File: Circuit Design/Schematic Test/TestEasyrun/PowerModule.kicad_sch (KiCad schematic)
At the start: 33 parts

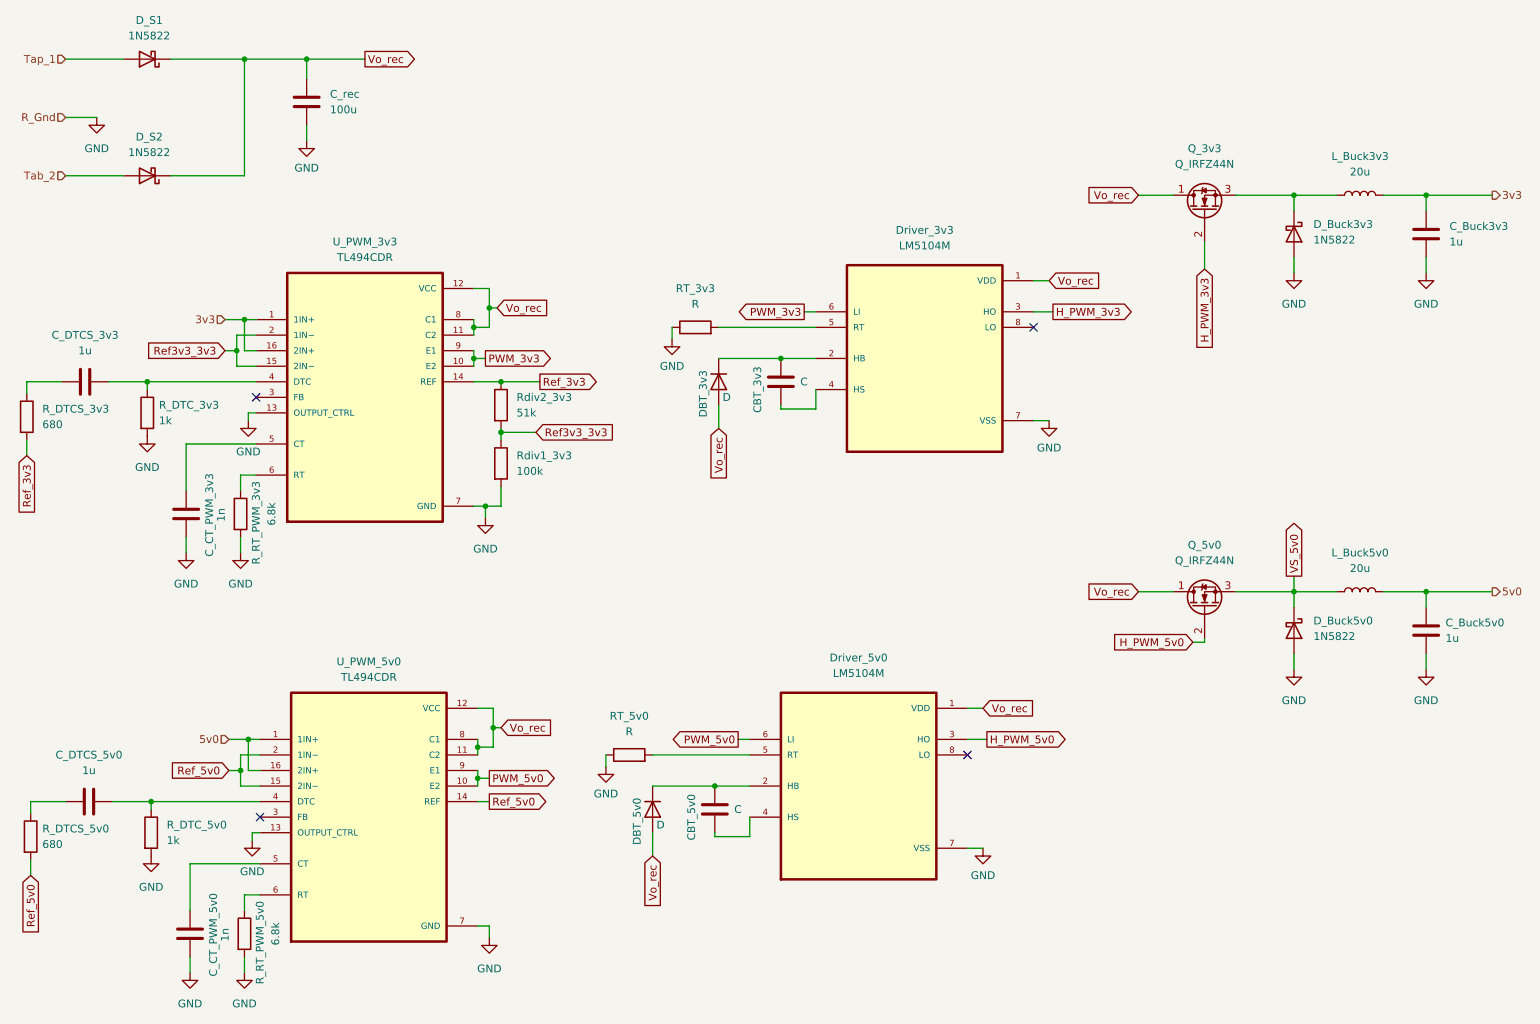
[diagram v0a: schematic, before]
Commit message: PWM generator file
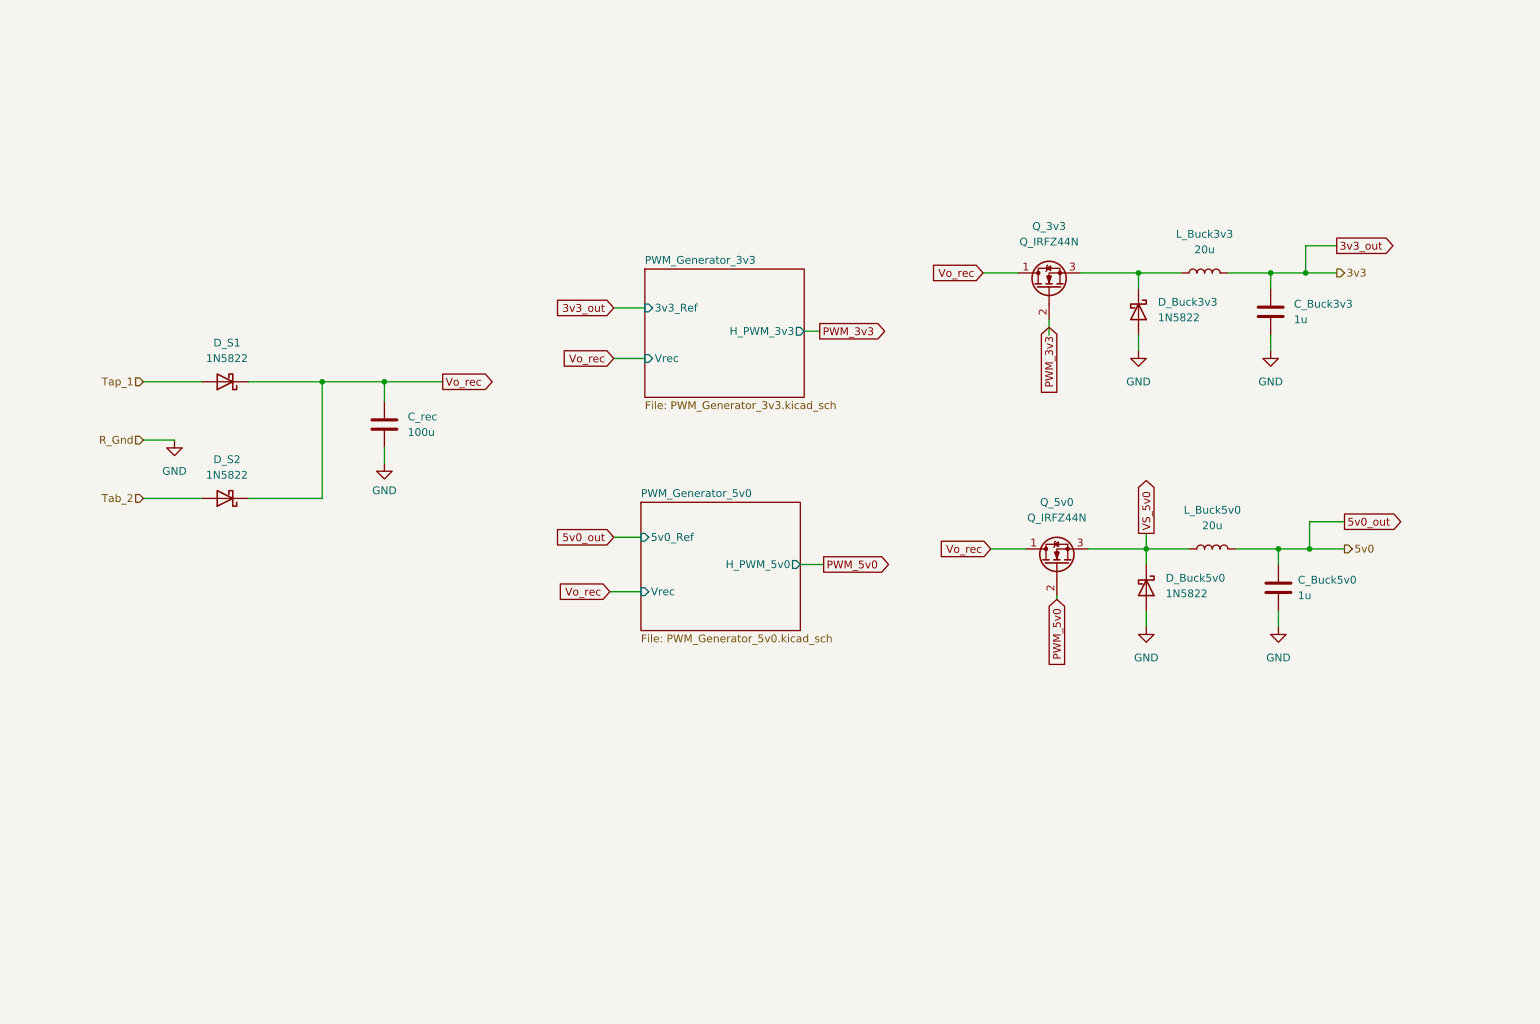
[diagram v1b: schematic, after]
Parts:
- removed CBT_3v3, CBT_5v0: C, Capacitor_SMD:C_0805_2012Metric_Pad1.18x1.45mm_HandSolder, symbol Device:C
- removed C_CT_PWM_3v3, C_CT_PWM_5v0: 1n, Capacitor_SMD:C_0805_2012Metric_Pad1.18x1.45mm_HandSolder, symbol Device:C
- removed C_DTCS_3v3, C_DTCS_5v0: 1u, Capacitor_SMD:C_0805_2012Metric_Pad1.18x1.45mm_HandSolder, symbol Device:C
- removed DBT_3v3, DBT_5v0: D, Diode_THT:D_DO-201AD_P15.24mm_Horizontal, symbol Device:D
- removed Driver_3v3, Driver_5v0: LM5104M, LM5104M:SOIC127P599X175-8N, symbol LM5104M:LM5104M
- removed RT_3v3, RT_5v0: R, Resistor_SMD:R_0805_2012Metric_Pad1.20x1.40mm_HandSolder, symbol Device:R
- removed R_DTCS_3v3, R_DTCS_5v0: 680, Resistor_SMD:R_0805_2012Metric_Pad1.20x1.40mm_HandSolder, symbol Device:R
- removed R_DTC_3v3, R_DTC_5v0: 1k, Resistor_SMD:R_0805_2012Metric_Pad1.20x1.40mm_HandSolder, symbol Device:R
- removed R_RT_PWM_3v3, R_RT_PWM_5v0: 6.8k, Resistor_SMD:R_0805_2012Metric_Pad1.20x1.40mm_HandSolder, symbol Device:R
- removed Rdiv1_3v3: 100k, Resistor_SMD:R_0805_2012Metric_Pad1.20x1.40mm_HandSolder, symbol Device:R
- removed Rdiv2_3v3: 51k, Resistor_SMD:R_0805_2012Metric_Pad1.20x1.40mm_HandSolder, symbol Device:R
- removed U_PWM_3v3, U_PWM_5v0: TL494CDR, TL494CDR_PWM:SOIC127P600X175-16N, symbol TL494CDR:TL494CDR
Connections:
- net H_PWM_3v3 is gone; now on net PWM_3v3: Q_3v3.2 (G)
- net H_PWM_5v0 is gone; now on net PWM_5v0: Q_5v0.2 (G)
- net 3v3 renamed 3v3_out
- net 5v0 renamed 5v0_out
- no-connect marks 4 -> 0
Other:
- added sheet PWM_Generator_3v3 (PWM_Generator_3v3.kicad_sch)
- added sheet PWM_Generator_5v0 (PWM_Generator_5v0.kicad_sch)
- moved on the sheet: C_Buck3v3, C_Buck5v0, C_rec, D_Buck3v3, D_Buck5v0, D_S1, D_S2, L_Buck3v3, L_Buck5v0, Q_3v3, Q_5v0
